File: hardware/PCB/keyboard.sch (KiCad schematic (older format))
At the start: 0 parts

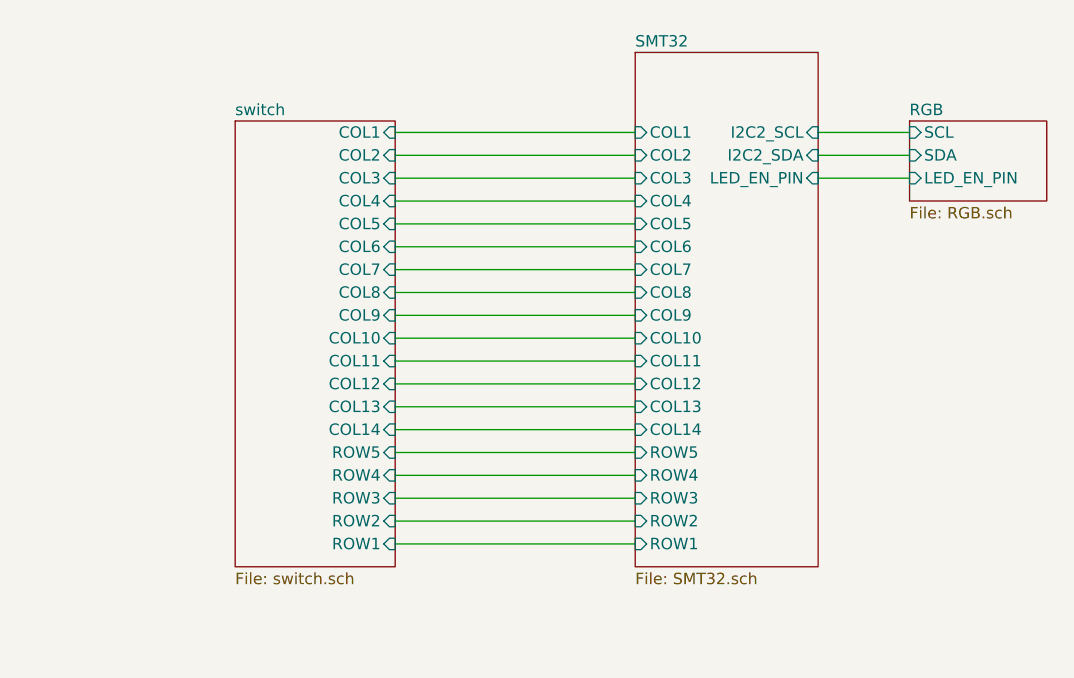
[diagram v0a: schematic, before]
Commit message: clear all the traces
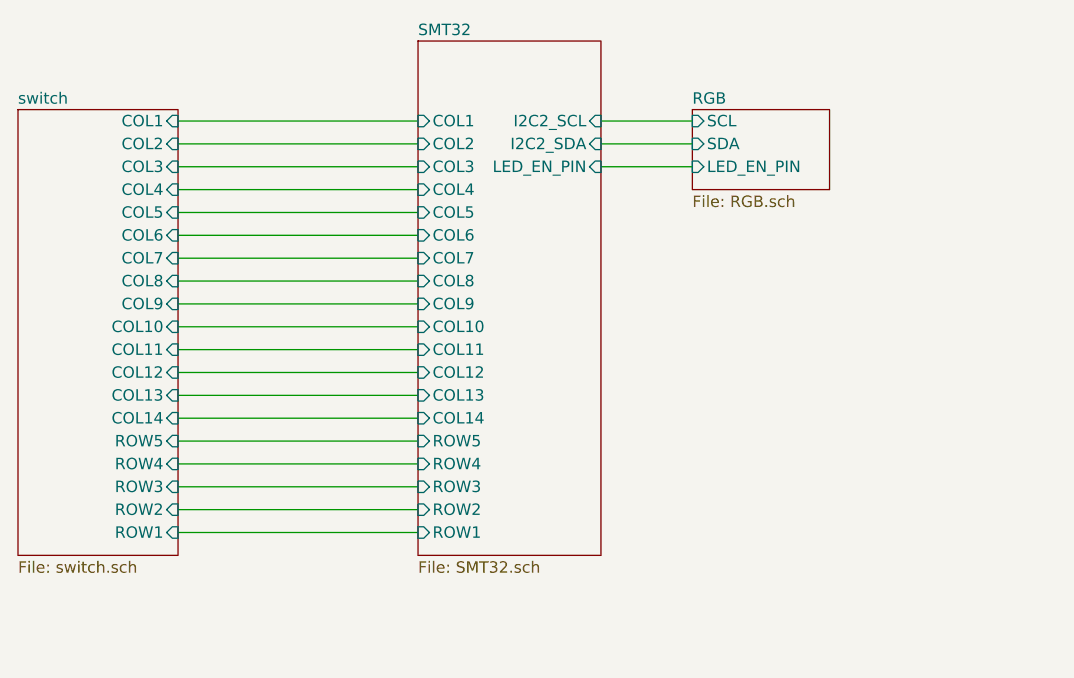
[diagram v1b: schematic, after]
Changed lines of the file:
@@
 $EndDescr
 $Sheet
-S 4700 2800 700  1950
+S 3750 2750 700  1950
 U 5E25E984
 F0 "switch" 50
 F1 "switch.sch" 50
-F2 "ROW1" I R 5400 4650 50
-F3 "ROW2" I R 5400 4550 50
-F4 "ROW3" I R 5400 4450 50
-F5 "ROW4" I R 5400 4350 50
-F6 "ROW5" I R 5400 4250 50
-F7 "COL1" I R 5400 2850 50
-F8 "COL2" I R 5400 2950 50
-F9 "COL3" I R 5400 3050 50
-F10 "COL4" I R 5400 3150 50
-F11 "COL5" I R 5400 3250 50
-F12 "COL6" I R 5400 3350 50
-F13 "COL7" I R 5400 3450 50
-F14 "COL8" I R 5400 3550 50
-F15 "COL9" I R 5400 3650 50
-F16 "COL10" I R 5400 3750 50
-F17 "COL11" I R 5400 3850 50
-F18 "COL12" I R 5400 3950 50
-F19 "COL13" I R 5400 4050 50
-F20 "COL14" I R 5400 4150 50
+F2 "ROW1" I R 4450 4600 50
+F3 "ROW2" I R 4450 4500 50
+F4 "ROW3" I R 4450 4400 50
+F5 "ROW4" I R 4450 4300 50
+F6 "ROW5" I R 4450 4200 50
+F7 "COL1" I R 4450 2800 50
+F8 "COL2" I R 4450 2900 50
+F9 "COL3" I R 4450 3000 50
+F10 "COL4" I R 4450 3100 50
+F11 "COL5" I R 4450 3200 50
+F12 "COL6" I R 4450 3300 50
+F13 "COL7" I R 4450 3400 50
+F14 "COL8" I R 4450 3500 50
+F15 "COL9" I R 4450 3600 50
+F16 "COL10" I R 4450 3700 50
+F17 "COL11" I R 4450 3800 50
+F18 "COL12" I R 4450 3900 50
+F19 "COL13" I R 4450 4000 50
+F20 "COL14" I R 4450 4100 50
 $EndSheet
 $Sheet
-S 7650 2800 600  350
+S 6700 2750 600  350
 U 5EC33E3D
 F0 "RGB" 50
 F1 "RGB.sch" 50
-F2 "SCL" I L 7650 2850 50
-F3 "SDA" I L 7650 2950 50
-F4 "LED_EN_PIN" I L 7650 3050 50
+F2 "SCL" I L 6700 2800 50
+F3 "SDA" I L 6700 2900 50
+F4 "LED_EN_PIN" I L 6700 3000 50
 $EndSheet
 $Sheet
-S 6450 2500 800  2250
+S 5500 2450 800  2250
 U 5E1424B2
 F0 "SMT32" 50
 F1 "SMT32.sch" 50
-F2 "I2C2_SDA" I R 7250 2950 50
-F3 "I2C2_SCL" I R 7250 2850 50
-F4 "COL1" I L 6450 2850 50
-F5 "COL2" I L 6450 2950 50
-F6 "COL3" I L 6450 3050 50
-F7 "COL4" I L 6450 3150 50
-F8 "COL5" I L 6450 3250 50
-F9 "COL6" I L 6450 3350 50
-F10 "COL7" I L 6450 3450 50
-F11 "COL8" I L 6450 3550 50
-F12 "COL9" I L 6450 3650 50
-F13 "COL10" I L 6450 3750 50
-F14 "COL11" I L 6450 3850 50
-F15 "COL12" I L 6450 3950 50
-F16 "COL13" I L 6450 4050 50
-F17 "COL14" I L 6450 4150 50
-F18 "ROW5" I L 6450 4250 50
-F19 "ROW4" I L 6450 4350 50
-F20 "ROW3" I L 6450 4450 50
-F21 "ROW2" I L 6450 4550 50
-F22 "ROW1" I L 6450 4650 50
-F23 "LED_EN_PIN" I R 7250 3050 50
+F2 "I2C2_SDA" I R 6300 2900 50
+F3 "I2C2_SCL" I R 6300 2800 50
+F4 "COL1" I L 5500 2800 50
+F5 "COL2" I L 5500 2900 50
+F6 "COL3" I L 5500 3000 50
+F7 "COL4" I L 5500 3100 50
+F8 "COL5" I L 5500 3200 50
+F9 "COL6" I L 5500 3300 50
+F10 "COL7" I L 5500 3400 50
+F11 "COL8" I L 5500 3500 50
+F12 "COL9" I L 5500 3600 50
+F13 "COL10" I L 5500 3700 50
+F14 "COL11" I L 5500 3800 50
+F15 "COL12" I L 5500 3900 50
+F16 "COL13" I L 5500 4000 50
+F17 "COL14" I L 5500 4100 50
+F18 "ROW5" I L 5500 4200 50
+F19 "ROW4" I L 5500 4300 50
+F20 "ROW3" I L 5500 4400 50
+F21 "ROW2" I L 5500 4500 50
+F22 "ROW1" I L 5500 4600 50
+F23 "LED_EN_PIN" I R 6300 3000 50
 $EndSheet
 Wire Wire Line
-	7250 2850 7650 2850
+	6300 2800 6700 2800
 Wire Wire Line
-	7650 2950 7250 2950
+	6700 2900 6300 2900
 Wire Wire Line
-	7250 3050 7650 3050
+	6300 3000 6700 3000
 Wire Wire Line
-	6450 2850 5400 2850
+	5500 2800 4450 2800
 Wire Wire Line
-	5400 2950 6450 2950
+	4450 2900 5500 2900
 Wire Wire Line
-	6450 3050 5400 3050
+	5500 3000 4450 3000
 Wire Wire Line
-	5400 3150 6450 3150
+	4450 3100 5500 3100
 Wire Wire Line
-	6450 3250 5400 3250
+	5500 3200 4450 3200
 Wire Wire Line
-	5400 3350 6450 3350
+	4450 3300 5500 3300
 Wire Wire Line
-	6450 3450 5400 3450
+	5500 3400 4450 3400
 Wire Wire Line
-	5400 3550 6450 3550
+	4450 3500 5500 3500
 Wire Wire Line
-	6450 3650 5400 3650
+	5500 3600 4450 3600
 Wire Wire Line
-	5400 3750 6450 3750
+	4450 3700 5500 3700
 Wire Wire Line
-	6450 3850 5400 3850
+	5500 3800 4450 3800
 Wire Wire Line
-	5400 3950 6450 3950
+	4450 3900 5500 3900
 Wire Wire Line
-	6450 4050 5400 4050
+	5500 4000 4450 4000
 Wire Wire Line
-	5400 4150 6450 4150
+	4450 4100 5500 4100
 Wire Wire Line
-	6450 4250 5400 4250
+	5500 4200 4450 4200
 Wire Wire Line
-	5400 4350 6450 4350
+	4450 4300 5500 4300
 Wire Wire Line
-	6450 4450 5400 4450
+	5500 4400 4450 4400
 Wire Wire Line
-	5400 4550 6450 4550
+	4450 4500 5500 4500
 Wire Wire Line
-	6450 4650 5400 4650
+	5500 4600 4450 4600
 $EndSCHEMATC

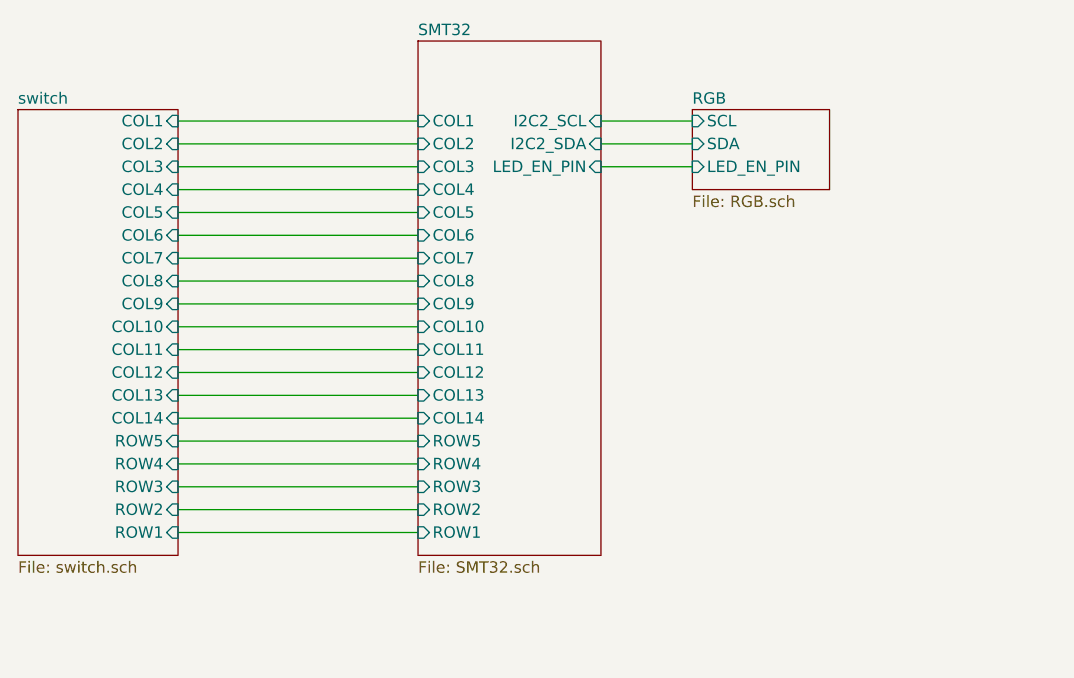
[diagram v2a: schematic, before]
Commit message: making progress
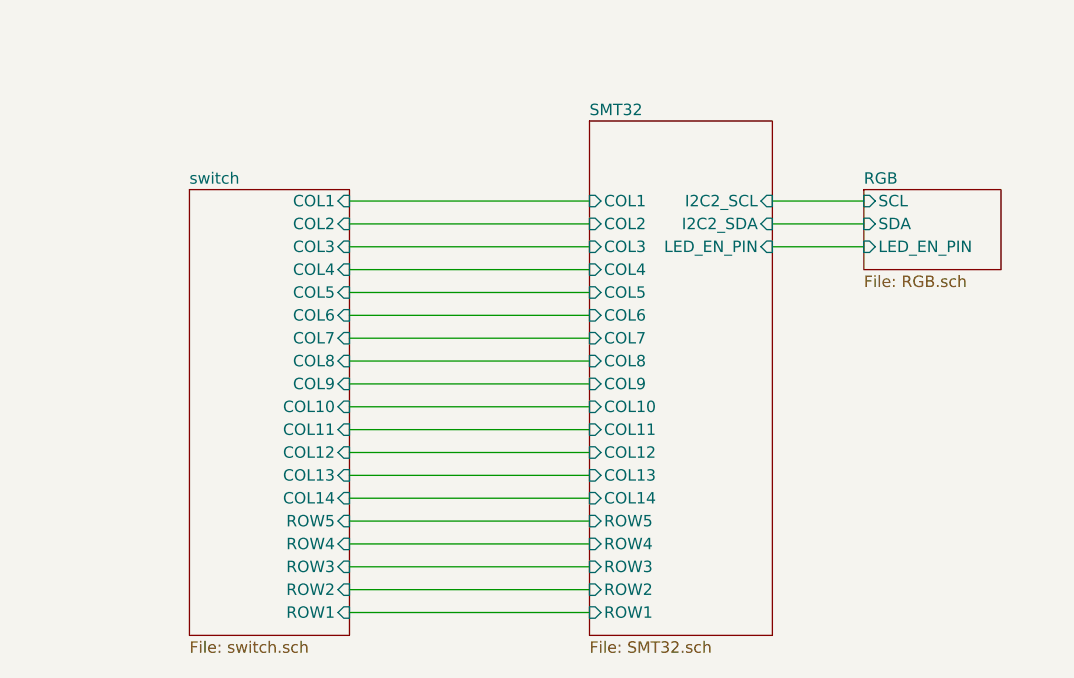
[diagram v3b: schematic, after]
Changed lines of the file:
@@
 $EndDescr
 $Sheet
-S 3750 2750 700  1950
+S 4500 3100 700  1950
 U 5E25E984
 F0 "switch" 50
 F1 "switch.sch" 50
-F2 "ROW1" I R 4450 4600 50
-F3 "ROW2" I R 4450 4500 50
-F4 "ROW3" I R 4450 4400 50
-F5 "ROW4" I R 4450 4300 50
-F6 "ROW5" I R 4450 4200 50
-F7 "COL1" I R 4450 2800 50
-F8 "COL2" I R 4450 2900 50
-F9 "COL3" I R 4450 3000 50
-F10 "COL4" I R 4450 3100 50
-F11 "COL5" I R 4450 3200 50
-F12 "COL6" I R 4450 3300 50
-F13 "COL7" I R 4450 3400 50
-F14 "COL8" I R 4450 3500 50
-F15 "COL9" I R 4450 3600 50
-F16 "COL10" I R 4450 3700 50
-F17 "COL11" I R 4450 3800 50
-F18 "COL12" I R 4450 3900 50
-F19 "COL13" I R 4450 4000 50
-F20 "COL14" I R 4450 4100 50
+F2 "ROW1" I R 5200 4950 50
+F3 "ROW2" I R 5200 4850 50
+F4 "ROW3" I R 5200 4750 50
+F5 "ROW4" I R 5200 4650 50
+F6 "ROW5" I R 5200 4550 50
+F7 "COL1" I R 5200 3150 50
+F8 "COL2" I R 5200 3250 50
+F9 "COL3" I R 5200 3350 50
+F10 "COL4" I R 5200 3450 50
+F11 "COL5" I R 5200 3550 50
+F12 "COL6" I R 5200 3650 50
+F13 "COL7" I R 5200 3750 50
+F14 "COL8" I R 5200 3850 50
+F15 "COL9" I R 5200 3950 50
+F16 "COL10" I R 5200 4050 50
+F17 "COL11" I R 5200 4150 50
+F18 "COL12" I R 5200 4250 50
+F19 "COL13" I R 5200 4350 50
+F20 "COL14" I R 5200 4450 50
 $EndSheet
 $Sheet
-S 6700 2750 600  350
+S 7450 3100 600  350
 U 5EC33E3D
 F0 "RGB" 50
 F1 "RGB.sch" 50
-F2 "SCL" I L 6700 2800 50
-F3 "SDA" I L 6700 2900 50
-F4 "LED_EN_PIN" I L 6700 3000 50
+F2 "SCL" I L 7450 3150 50
+F3 "SDA" I L 7450 3250 50
+F4 "LED_EN_PIN" I L 7450 3350 50
 $EndSheet
 $Sheet
-S 5500 2450 800  2250
+S 6250 2800 800  2250
 U 5E1424B2
 F0 "SMT32" 50
 F1 "SMT32.sch" 50
-F2 "I2C2_SDA" I R 6300 2900 50
-F3 "I2C2_SCL" I R 6300 2800 50
-F4 "COL1" I L 5500 2800 50
-F5 "COL2" I L 5500 2900 50
-F6 "COL3" I L 5500 3000 50
-F7 "COL4" I L 5500 3100 50
-F8 "COL5" I L 5500 3200 50
-F9 "COL6" I L 5500 3300 50
-F10 "COL7" I L 5500 3400 50
-F11 "COL8" I L 5500 3500 50
-F12 "COL9" I L 5500 3600 50
-F13 "COL10" I L 5500 3700 50
-F14 "COL11" I L 5500 3800 50
-F15 "COL12" I L 5500 3900 50
-F16 "COL13" I L 5500 4000 50
-F17 "COL14" I L 5500 4100 50
-F18 "ROW5" I L 5500 4200 50
-F19 "ROW4" I L 5500 4300 50
-F20 "ROW3" I L 5500 4400 50
-F21 "ROW2" I L 5500 4500 50
-F22 "ROW1" I L 5500 4600 50
-F23 "LED_EN_PIN" I R 6300 3000 50
+F2 "I2C2_SDA" I R 7050 3250 50
+F3 "I2C2_SCL" I R 7050 3150 50
+F4 "COL1" I L 6250 3150 50
+F5 "COL2" I L 6250 3250 50
+F6 "COL3" I L 6250 3350 50
+F7 "COL4" I L 6250 3450 50
+F8 "COL5" I L 6250 3550 50
+F9 "COL6" I L 6250 3650 50
+F10 "COL7" I L 6250 3750 50
+F11 "COL8" I L 6250 3850 50
+F12 "COL9" I L 6250 3950 50
+F13 "COL10" I L 6250 4050 50
+F14 "COL11" I L 6250 4150 50
+F15 "COL12" I L 6250 4250 50
+F16 "COL13" I L 6250 4350 50
+F17 "COL14" I L 6250 4450 50
+F18 "ROW5" I L 6250 4550 50
+F19 "ROW4" I L 6250 4650 50
+F20 "ROW3" I L 6250 4750 50
+F21 "ROW2" I L 6250 4850 50
+F22 "ROW1" I L 6250 4950 50
+F23 "LED_EN_PIN" I R 7050 3350 50
 $EndSheet
 Wire Wire Line
-	6300 2800 6700 2800
+	7050 3150 7450 3150
 Wire Wire Line
-	6700 2900 6300 2900
+	7450 3250 7050 3250
 Wire Wire Line
-	6300 3000 6700 3000
+	7050 3350 7450 3350
 Wire Wire Line
-	5500 2800 4450 2800
+	6250 3150 5200 3150
 Wire Wire Line
-	4450 2900 5500 2900
+	5200 3250 6250 3250
 Wire Wire Line
-	5500 3000 4450 3000
+	6250 3350 5200 3350
 Wire Wire Line
-	4450 3100 5500 3100
+	5200 3450 6250 3450
 Wire Wire Line
-	5500 3200 4450 3200
+	6250 3550 5200 3550
 Wire Wire Line
-	4450 3300 5500 3300
+	5200 3650 6250 3650
 Wire Wire Line
-	5500 3400 4450 3400
+	6250 3750 5200 3750
 Wire Wire Line
-	4450 3500 5500 3500
+	5200 3850 6250 3850
 Wire Wire Line
-	5500 3600 4450 3600
+	6250 3950 5200 3950
 Wire Wire Line
-	4450 3700 5500 3700
+	5200 4050 6250 4050
 Wire Wire Line
-	5500 3800 4450 3800
+	6250 4150 5200 4150
 Wire Wire Line
-	4450 3900 5500 3900
+	5200 4250 6250 4250
 Wire Wire Line
-	5500 4000 4450 4000
+	6250 4350 5200 4350
 Wire Wire Line
-	4450 4100 5500 4100
+	5200 4450 6250 4450
 Wire Wire Line
-	5500 4200 4450 4200
+	6250 4550 5200 4550
 Wire Wire Line
-	4450 4300 5500 4300
+	5200 4650 6250 4650
 Wire Wire Line
-	5500 4400 4450 4400
+	6250 4750 5200 4750
 Wire Wire Line
-	4450 4500 5500 4500
+	5200 4850 6250 4850
 Wire Wire Line
-	5500 4600 4450 4600
+	6250 4950 5200 4950
 $EndSCHEMATC
